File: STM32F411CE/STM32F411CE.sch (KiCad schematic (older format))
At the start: 16 parts, among them J1 USB_B_Mini, J2 Conn_01x20_Male, J3 Conn_01x20_Male, U2 USBLC6-2SC6, U3 STM32F411CEUx, Y1 Crystal_GND24

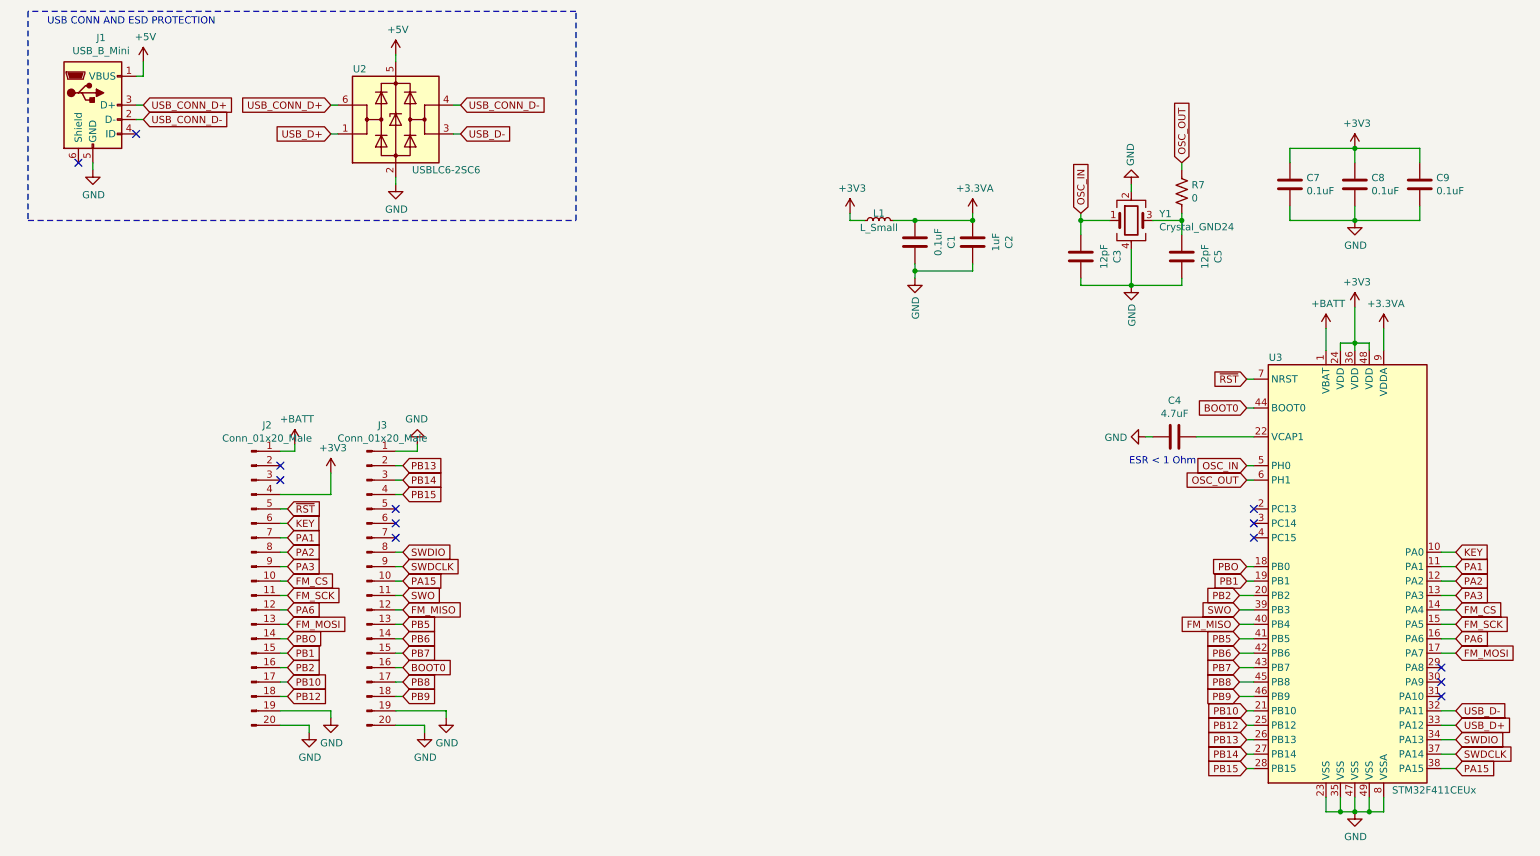
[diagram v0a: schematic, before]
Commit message: finish off the stm32f411ce
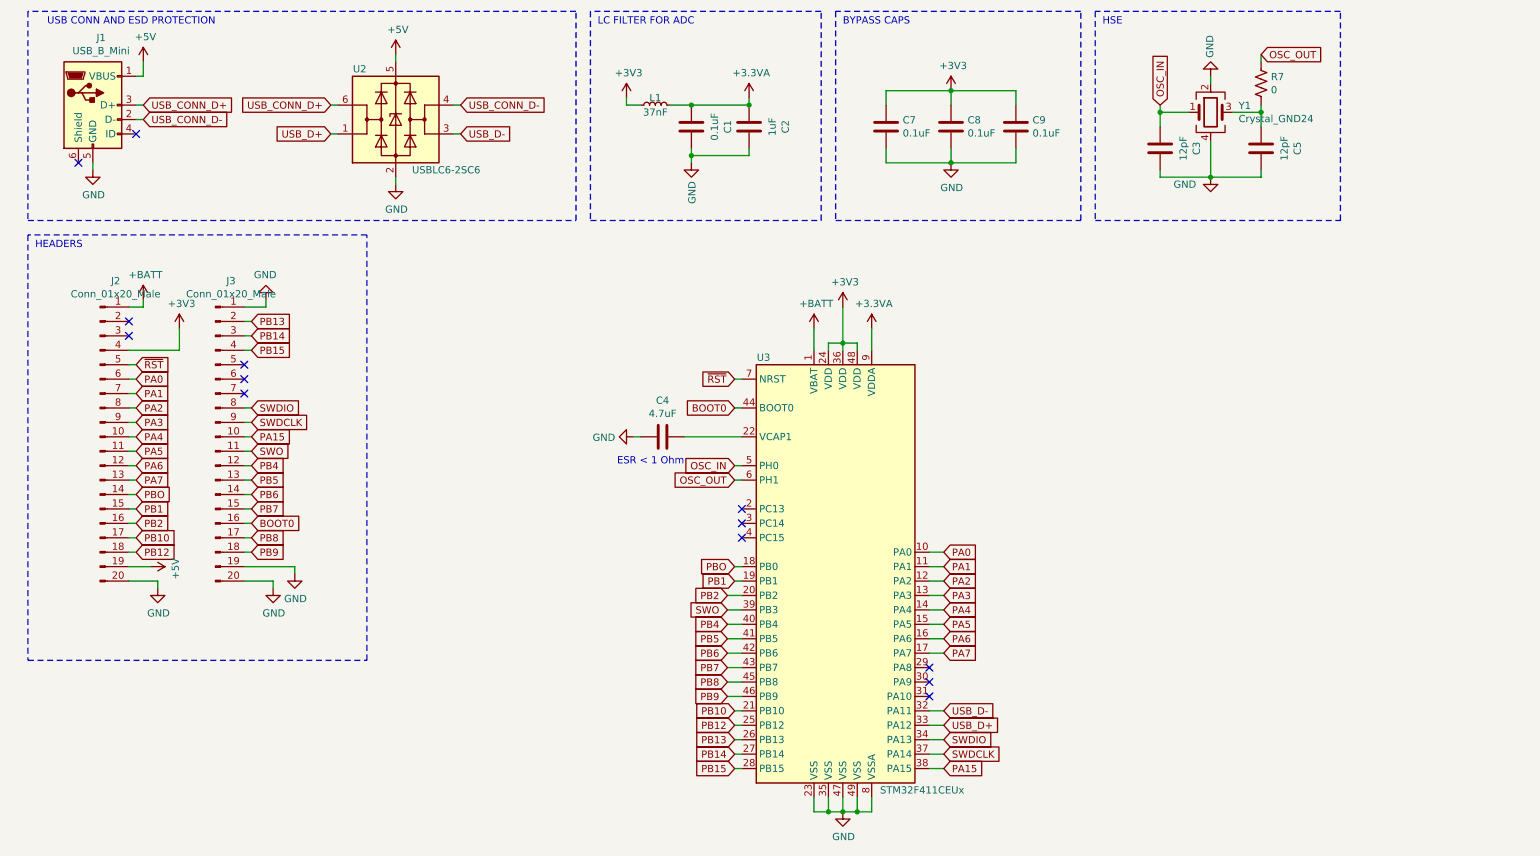
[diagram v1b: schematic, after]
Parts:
- L1: value L_Small -> 37nF
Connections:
- net +5V: now also J2.19 (Pin_19)
- net GND: no longer J2.19 (Pin_19)
- net FM_CS renamed PA4
- net FM_MISO renamed PB4
- net FM_MOSI renamed PA7
- net FM_SCK renamed PA5
- net KEY renamed PA0
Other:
- note added: "BYPASS CAPS"
- note added: "HEADERS"
- note added: "HSE"
- note added: "LC FILTER FOR ADC"
- moved on the sheet: C1, C2, C3, C4, C5, C7, C8, C9, J2, J3, L1, R7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
